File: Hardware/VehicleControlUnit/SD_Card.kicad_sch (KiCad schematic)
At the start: 6 parts, among them J12 Micro_SD_Card_Det2

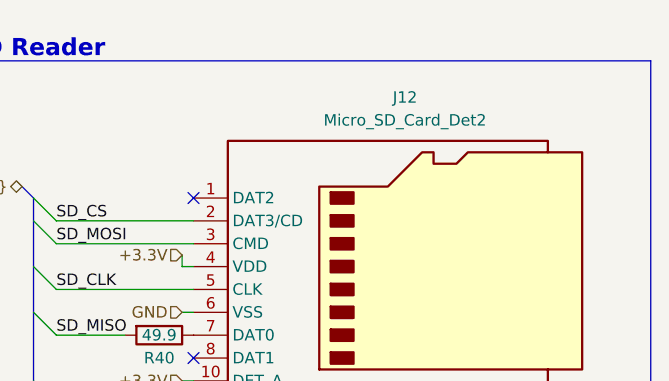
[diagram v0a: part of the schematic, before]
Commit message: VCU hardware prod files done night night
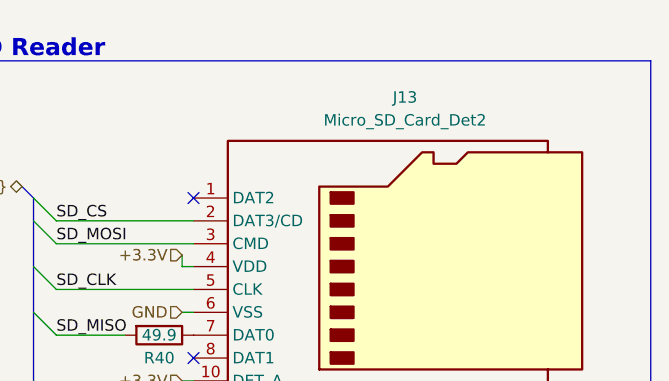
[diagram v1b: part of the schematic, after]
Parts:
- renumbered J12 to J13
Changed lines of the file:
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@@
 		(dnp no)
 		(fields_autoplaced yes)
-		(property "Reference" "J12"
+		(property "Reference" "J13"
 			(at 155.575 43.434 0)
 			(show_name no)
@@
 			(project "VehicleControlUnit"
 				(path "/e864fac9-3897-46c9-9101-6d5488c6cd3a/b0b52d73-b085-4624-9871-af1c22d24972"
-					(reference "J12")
+					(reference "J13")
 					(unit 1)
 				)

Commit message: surabhi review pls
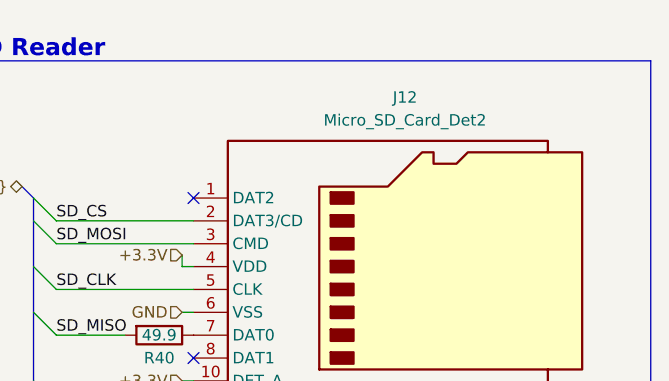
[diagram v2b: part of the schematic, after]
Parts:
- renumbered J13 to J12
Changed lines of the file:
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@@
 		(dnp no)
 		(fields_autoplaced yes)
-		(property "Reference" "J13"
+		(property "Reference" "J12"
 			(at 155.575 43.434 0)
 			(show_name no)
@@
 			(project "VehicleControlUnit"
 				(path "/e864fac9-3897-46c9-9101-6d5488c6cd3a/b0b52d73-b085-4624-9871-af1c22d24972"
-					(reference "J13")
+					(reference "J12")
 					(unit 1)
 				)
